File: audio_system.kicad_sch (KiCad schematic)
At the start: 8 parts, among them U2 MCP4725xxx-xCH, U3 MAX98306xDT

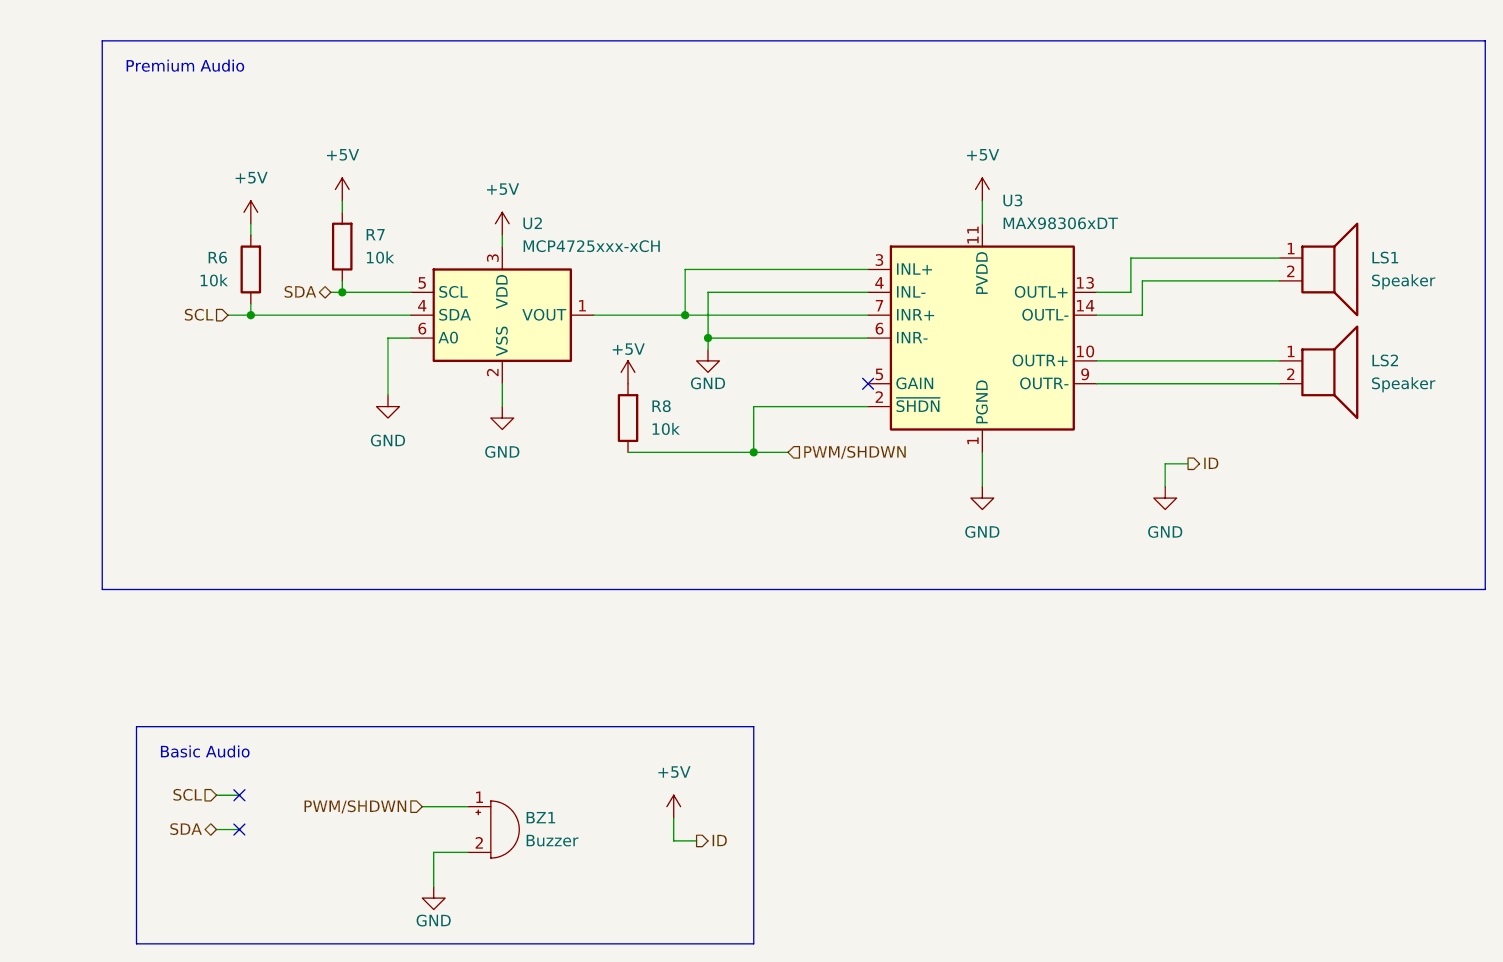
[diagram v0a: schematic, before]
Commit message: Finalized Schematic
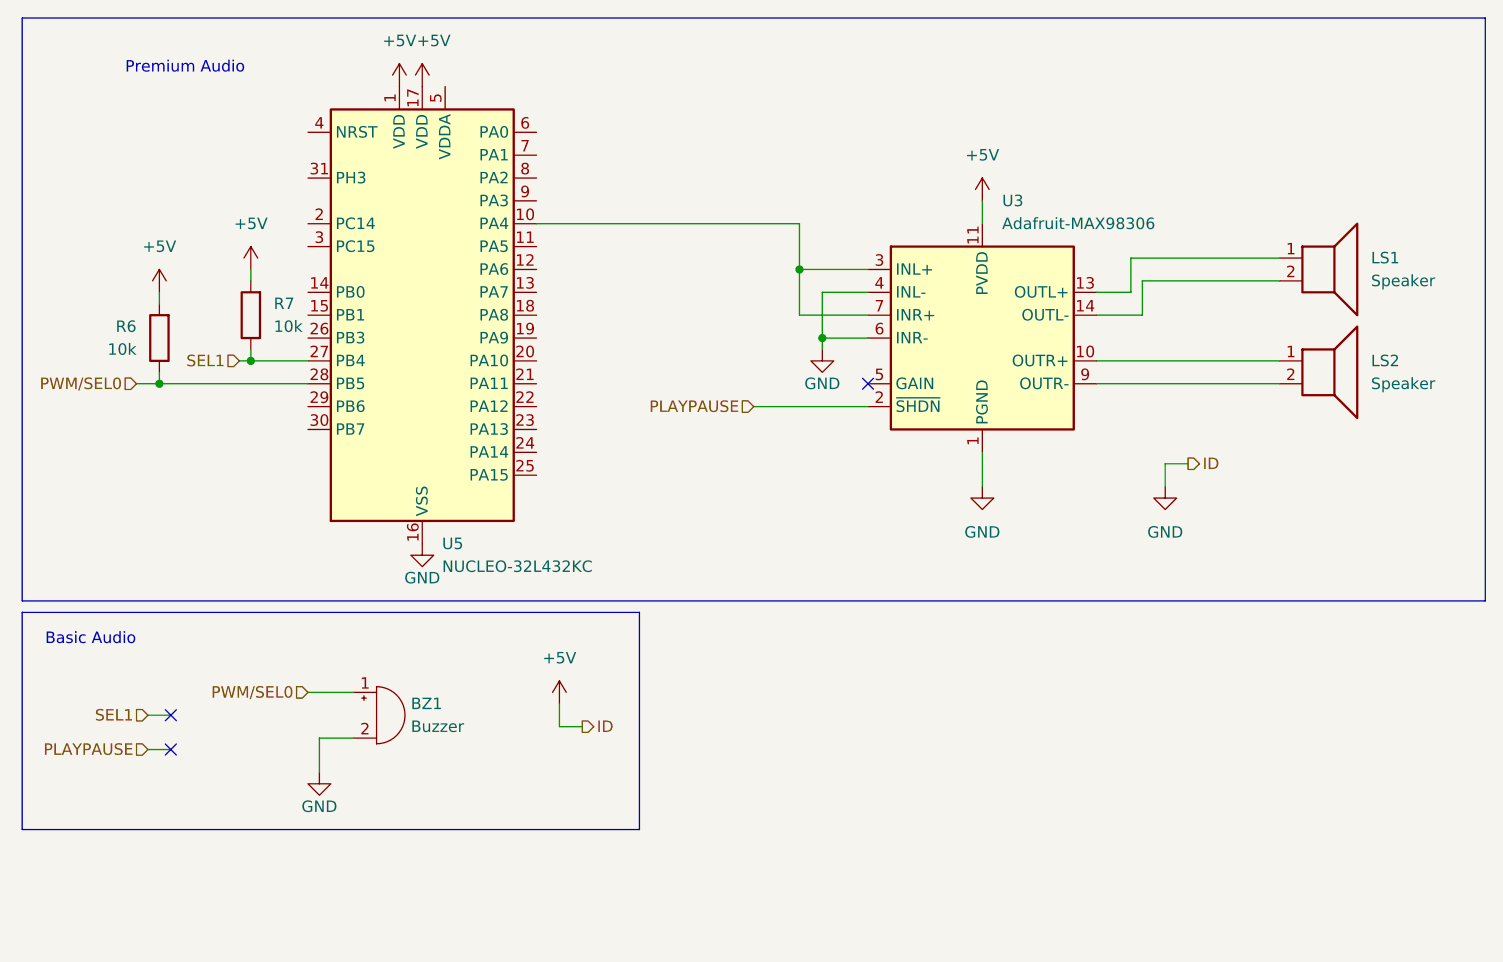
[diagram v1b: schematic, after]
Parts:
- removed R8: 10k, symbol Device:R
- removed U2: MCP4725xxx-xCH, Package_TO_SOT_SMD:SOT-23-6, symbol Analog_DAC:MCP4725xxx-xCH
- added U5: NUCLEO-32L432KC, Package_DFN_QFN:QFN-32-1EP_5x5mm_P0.5mm_EP3.45x3.45mm, symbol MCU_ST_STM32L4:STM32L432KBUx
- U3: value MAX98306xDT -> Adafruit-MAX98306
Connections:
- net +5V: now also U5.1 (VDD), U5.16 (VSS), U5.17 (VDD), U5.32 (VSS), U5.33 (VSS)
- net at U3.3 (INL+), U3.7 (INR+): now also U5.10 (PA4)
- net PWM/SHDWN renamed PLAYPAUSE
- net PLAYPAUSE: no longer BZ1.1 (-)
- net SCL renamed PWM/SEL0
- net PWM/SEL0: now also BZ1.1 (-), U5.28 (PB5)
- net SDA renamed SEL1
- net SEL1: now also U5.27 (PB4)
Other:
- moved on the sheet: BZ1, R6, R7
